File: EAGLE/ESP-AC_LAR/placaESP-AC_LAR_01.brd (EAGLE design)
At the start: 42.5 x 44.5 mm, 13 parts, among them Q1 2N4401

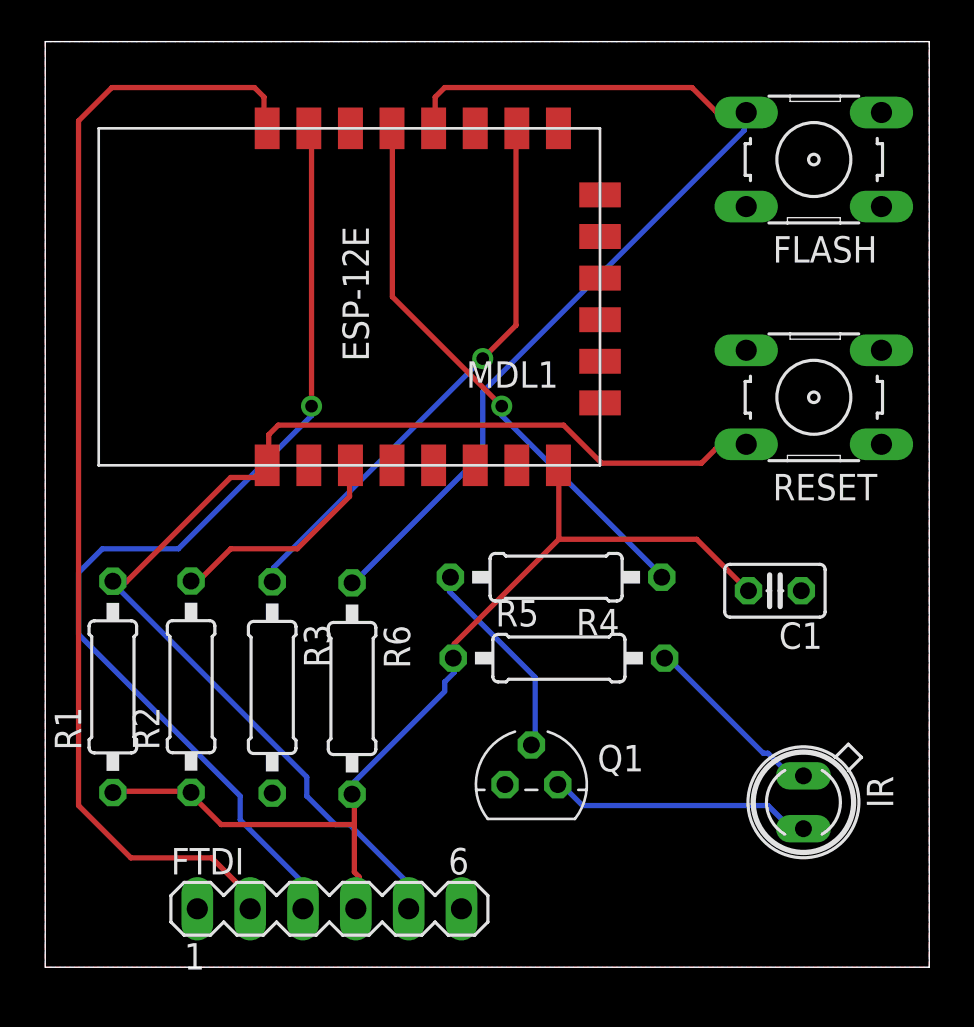
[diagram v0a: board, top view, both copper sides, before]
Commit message: Modificações - dia 03/02/17
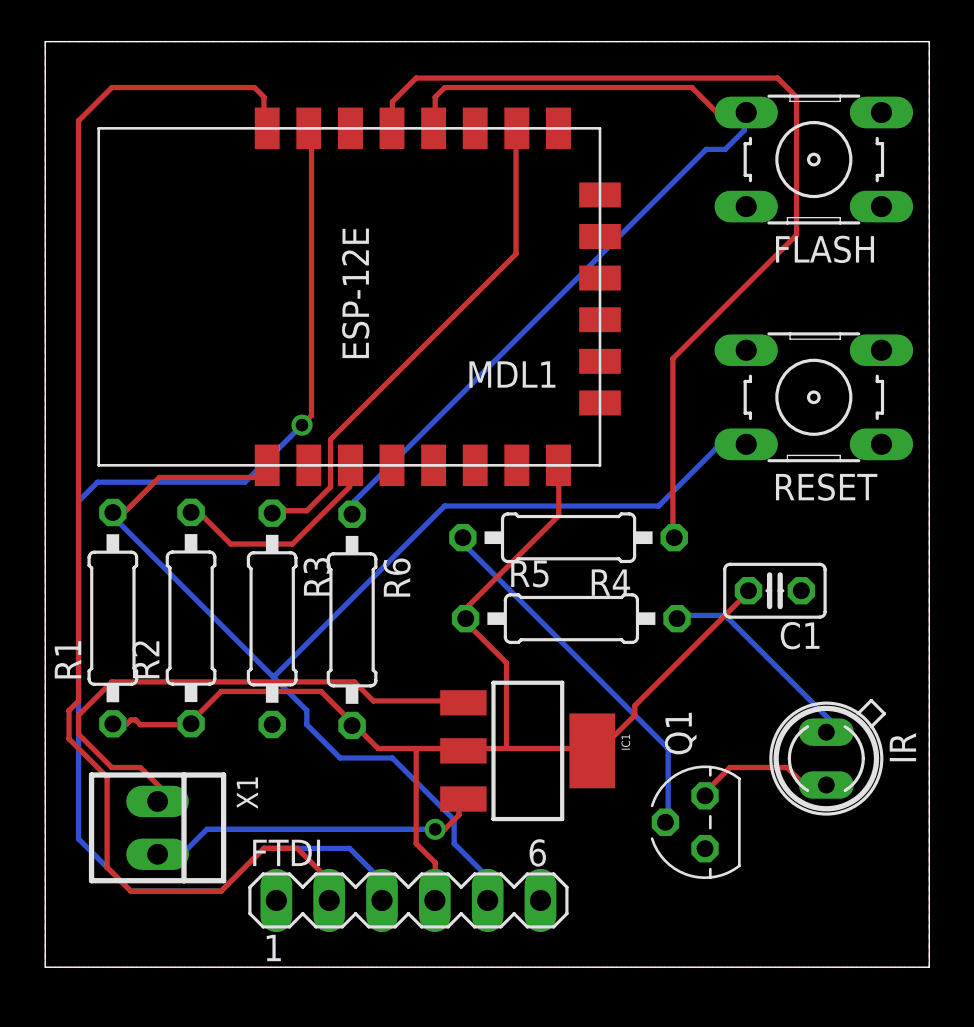
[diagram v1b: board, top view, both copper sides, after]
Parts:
- added IC1: (no value), kaibader:AMS1117
- added X1: 22-23-2021, con-molex:22-23-2021
- moved Q1 8.54 mm to (31.7, 6.97), turned to 90 degrees
- moved FTDI 3.82 mm to (17.5, 3.21)
- moved R2 3.30 mm to (7.01, 16.8)
- moved R3 3.30 mm to (10.9, 16.8)
- moved R1 3.30 mm to (3.25, 16.8)
- moved R6 3.30 mm to (14.8, 16.7)
- moved IR 2.37 mm to (37.5, 10.0)
- moved R5 1.99 mm to (25.3, 16.8)
- moved R4 1.99 mm to (25.2, 20.6)
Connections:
- new net IN+: IC1.VIN, X1.2
- new net IN-: IC1.GND, X1.1
- net VCC: now also IC1.HEATSINK, IC1.VOUT
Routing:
- net IN-: track 0.00 -> 26.2 mm
- net IO4: track 27.1 -> 45.2 mm, vias 1 -> 0
- net IN+: track 0.00 -> 16.2 mm, vias 0 -> 1
- net VCC: track 48.1 -> 60.7 mm
- net TXO: track 48.8 -> 61.1 mm
- net N$3: track 9.94 -> 18.0 mm
- net RXI: track 54.9 -> 61.8 mm
- net N$4: track 12.7 -> 6.86 mm
- net CTS: track 57.6 -> 63.4 mm
- net N$6: track 47.6 -> 44.8 mm
- net N$5: track 26.6 -> 24.3 mm, vias 1 -> 0
- net N$2: track 9.05 -> 10.2 mm
